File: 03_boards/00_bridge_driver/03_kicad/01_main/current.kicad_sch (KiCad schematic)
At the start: 25 parts, among them U10 TLV2371P, U11 INA241A2xD, U12 AMC1311, U13 AMC1311, U16 INA241A2xD

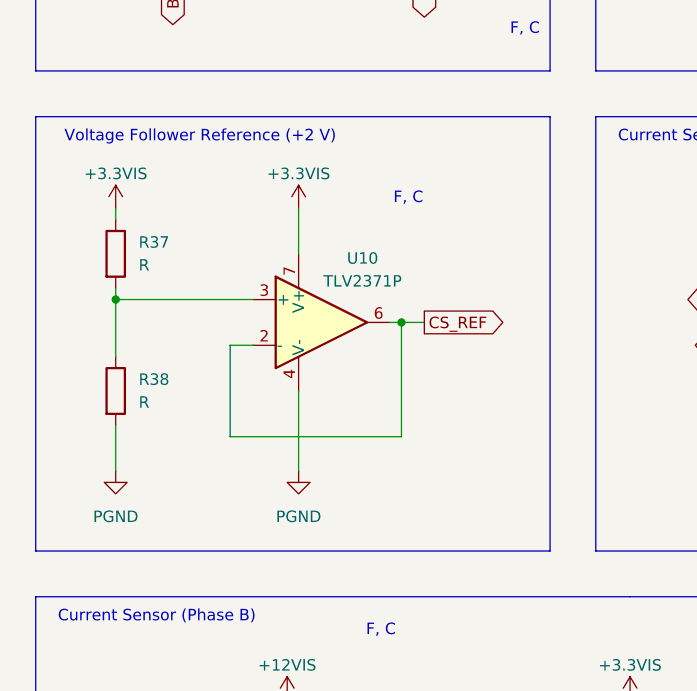
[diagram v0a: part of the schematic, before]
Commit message: Finished Driver Board Schematic.
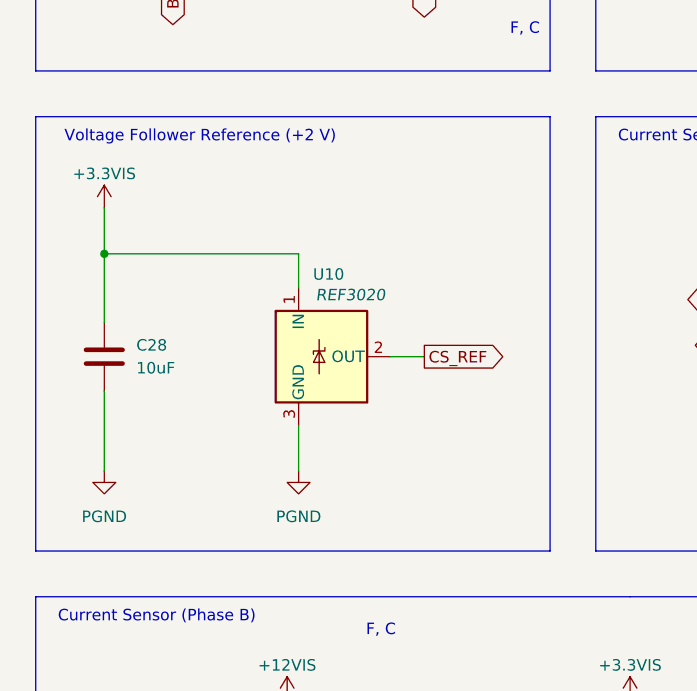
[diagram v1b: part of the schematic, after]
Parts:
- removed R37, R38: R, symbol Device:R
- removed U10: TLV2371P, Package_DIP:DIP-8_W7.62mm, symbol Amplifier_Operational:TLV2371P
- added C28: 10uF, symbol Device:C
- added U10: REF3020, Package_TO_SOT_SMD:SOT-23, symbol Reference_Voltage:REF3020
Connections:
- net +3.3VIS: now also C28.1, U10.1 (IN)
- net CS_REF: now also U10.2 (OUT)
- net PGND: now also C28.2, U10.3 (GND)
